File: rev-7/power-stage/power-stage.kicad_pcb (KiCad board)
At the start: 6 copper layers, 40 x 39.5 mm, 102 parts, among them J1 10132797-021100LF, J2 10132797-021100LF, J3 10132797-021100LF, J4 Motor, Q1 LMG5200, Q2 LMG5200, Q3 LMG5200, U1 AS5047P, U2 INA240A1PW, U3 INA240A1PW, U4 INA240A1PW

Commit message: Updating
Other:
- board text added: "Cutout GND plane under SW nodes"
- board text added: "F.Cu -> Sig In1.Cu -> PGND In2.Cu -> VBUS / sig In3.Cu -> Analog Sig In4.Cu -> PGND/GND B.Cu -> Phase/Sig"
- board text added: "Layer stackup: OSHPark 6-L 1oz copper -- 0.11mm prepreg -- 0.5oz copper -- 0.10mm prepreg -- 0.50oz copper -- 0.92mm core -- 0.5oz copper -- 0.10mm prepreg -- 0.5oz copper -- 0.11mm prepreg -- 1oz copper"
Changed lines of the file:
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@@
     (fp_line (start -15.000001 13.723079) (end -15.000001 13.435892) (layer "B.Mask") (width 0.1))
     (fp_line (start -14.000001 -14.276921) (end -16.890983 -14.276922) (layer "B.Mask") (width 0.1))
-    (fp_arc (start 16.890992 -14.276909) (mid 17.013752 -14.119771) (end 17.114589 -13.947741) (layer "B.Mask") (width 0.1))
+    (fp_arc (start 16.890992 -14.276909) (mid 17.013756 -14.119774) (end 17.114589 -13.947741) (layer "B.Mask") (width 0.1))
     (fp_arc (start -17.114591 -13.947741) (mid -17.013752 -14.11978) (end -16.890983 -14.276922) (layer "B.Mask") (width 0.1))
     (fp_arc (start -14.000001 14.723079) (mid -14.707108 14.430186) (end -15.000001 13.723079) (layer "B.Mask") (width 0.1))
@@
       (connect_pads (clearance 0))
       (min_thickness 0.254)
-      (keepout (tracks allowed) (vias allowed) (pads not_allowed ) (copperpour allowed) (footprints not_allowed))
+      (keepout (tracks allowed) (vias allowed) (pads not_allowed) (copperpour allowed) (footprints not_allowed))
       (fill (thermal_gap 0.508) (thermal_bridge_width 0.508))
       (polygon
@@
       (connect_pads (clearance 0))
       (min_thickness 0.254)
-      (keepout (tracks allowed) (vias allowed) (pads not_allowed ) (copperpour allowed) (footprints not_allowed))
+      (keepout (tracks allowed) (vias allowed) (pads not_allowed) (copperpour allowed) (footprints not_allowed))
       (fill (thermal_gap 0.508) (thermal_bridge_width 0.508))
       (polygon
@@
     )
   )
+  (gr_text "Layer stackup:\nOSHPark 6-L\n1oz copper\n-- 0.11mm prepreg --\n0.5oz copper\n-- 0.10mm prepreg --\n0.50oz copper\n-- 0.92mm core -- \n0.5oz copper \n-- 0.10mm prepreg --\n0.5oz copper\n-- 0.11mm prepreg --\n1oz copper" (at 128.15 51.45) (layer "Cmts.User")
+    (effects (font (size 0.5 0.5) (thickness 0.1)))
+  )
   (gr_text "1.65mm Clearance Zone" (at 97.475 62.425) (layer "Cmts.User")
     (effects (font (size 0.6 0.6) (thickness 0.15)))
   )
+  (gr_text "F.Cu -> Sig\nIn1.Cu -> PGND\nIn2.Cu -> VBUS / sig\nIn3.Cu -> Analog Sig\nIn4.Cu -> PGND/GND\nB.Cu -> Phase/Sig" (at 125.65 67.4) (layer "Cmts.User")
+    (effects (font (size 0.5 0.5) (thickness 0.1)))
+  )
+  (gr_text "Cutout GND plane under SW nodes" (at 127.2 74.4) (layer "Cmts.User")
+    (effects (font (size 0.5 0.5) (thickness 0.1)))
+  )
   (zone (net 43) (net_name "/PHA_RAW") (layer "F.Cu") (hatch edge 0.508)

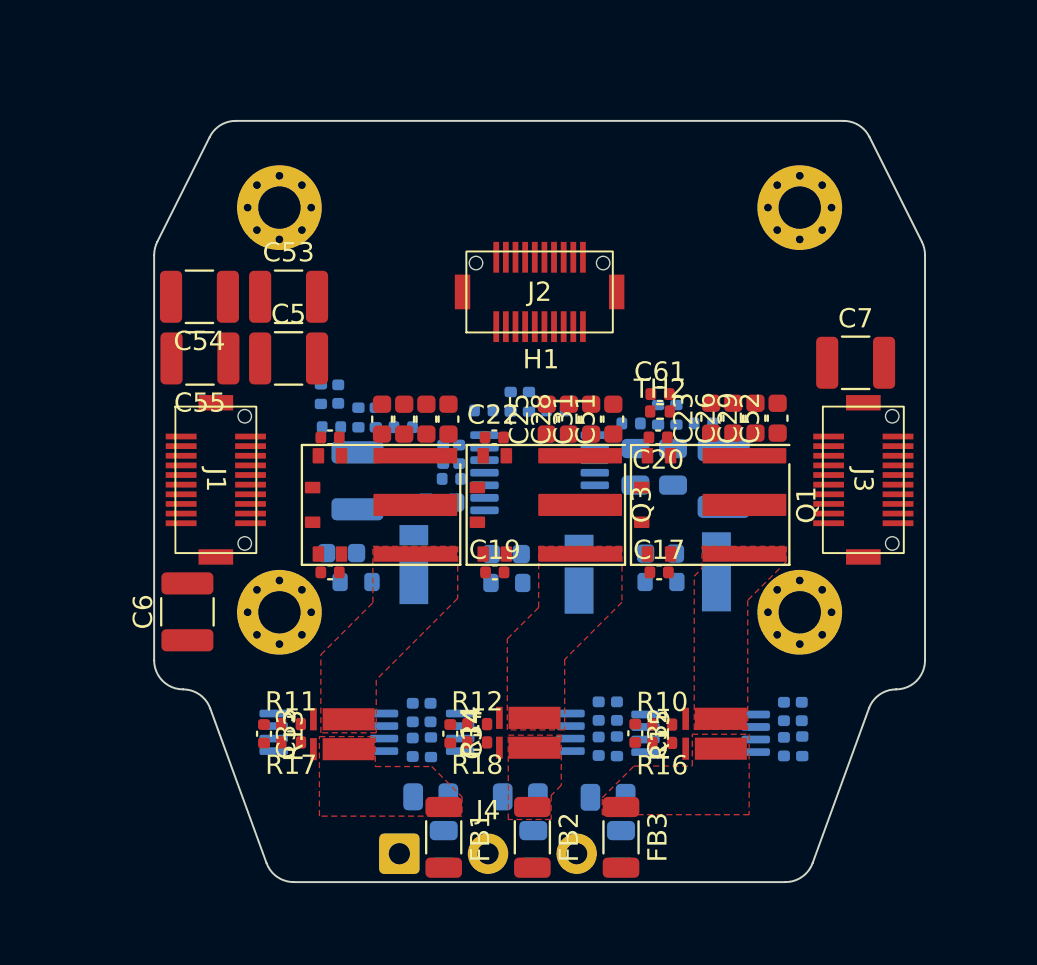
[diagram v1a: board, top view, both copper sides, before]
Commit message: Rev 7 RC1 - Push before design review
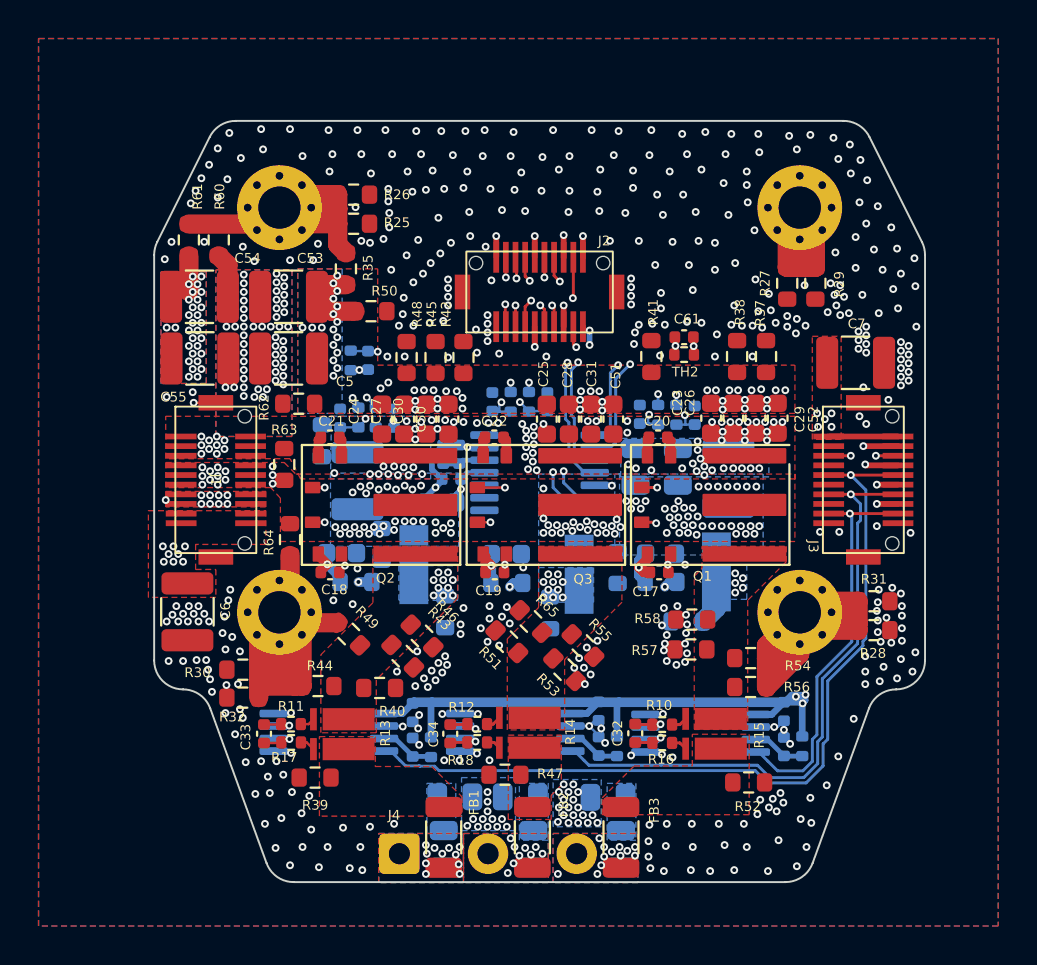
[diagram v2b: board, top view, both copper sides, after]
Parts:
- removed C44, C45, C46: 2.2u, Capacitor_SMD:C_0402_1005Metric
- added R25: THJP0603ABT1, Resistor_SMD:R_0603_1608Metric, F.Cu at (87.7, 54.5)
- added R26: THJP0603ABT1, Resistor_SMD:R_0603_1608Metric, F.Cu at (87.7, 53.0)
- added R27: THJP0603ABT1, Resistor_SMD:R_0603_1608Metric, F.Cu at (110.2, 57.5)
- added R28: THJP0603ABT1, Resistor_SMD:R_0603_1608Metric, F.Cu at (114.7, 75.5)
- added R29: THJP0603ABT1, Resistor_SMD:R_0603_1608Metric, F.Cu at (111.6, 57.5)
- added R30: THJP0603ABT1, Resistor_SMD:R_0603_1608Metric, F.Cu at (81.9, 77.6)
- added R31: THJP0603ABT1, Resistor_SMD:R_0603_1608Metric, F.Cu at (114.7, 74.0)
- added R32: THJP0603ABT1, Resistor_SMD:R_0603_1608Metric, F.Cu at (81.9, 79.0)
- added R33: THJP0603ABT1, Resistor_SMD:R_0603_1608Metric, B.Cu at (89.1, 71.1)
- added R34: THJP0603ABT1, Resistor_SMD:R_0603_1608Metric, B.Cu at (86.0, 65.7)
- added R35: THJP0603ABT1, Resistor_SMD:R_0603_1608Metric, F.Cu at (87.2, 56.8)
- added R36: THJP0603ABT1, Resistor_SMD:R_0603_1608Metric, B.Cu at (101.3, 72.3)
- added R37: THJP0603ABT1, Resistor_SMD:R_0603_1608Metric, F.Cu at (109.0, 61.4)
- added R38: THJP0603ABT1, Resistor_SMD:R_0603_1608Metric, F.Cu at (107.5, 61.4)
- added R39: THJP0603ABT1, Resistor_SMD:R_0603_1608Metric, F.Cu at (85.7, 83.2)
- added R40: THJP0603ABT1, Resistor_SMD:R_0603_1608Metric, F.Cu at (89.0, 78.5)
- added R41: THJP0603ABT1, Resistor_SMD:R_0603_1608Metric, F.Cu at (103.1, 61.4)
- added R42: THJP0603ABT1, Resistor_SMD:R_0603_1608Metric, F.Cu at (93.3, 61.4)
- added R43: THJP0603ABT1, Resistor_SMD:R_0603_1608Metric, F.Cu at (90.2, 76.9)
- added R44: THJP0603ABT1, Resistor_SMD:R_0603_1608Metric, F.Cu at (85.8, 78.5)
- added R45: THJP0603ABT1, Resistor_SMD:R_0603_1608Metric, F.Cu at (91.9, 61.4)
- added R46: THJP0603ABT1, Resistor_SMD:R_0603_1608Metric, F.Cu at (91.2, 75.8)
- added R47: THJP0603ABT1, Resistor_SMD:R_0603_1608Metric, F.Cu at (95.5, 83.0)
- added R48: THJP0603ABT1, Resistor_SMD:R_0603_1608Metric, F.Cu at (90.4, 61.4)
- added R49: THJP0603ABT1, Resistor_SMD:R_0603_1608Metric, F.Cu at (87.4, 75.8)
- added R50: THJP0603ABT1, Resistor_SMD:R_0603_1608Metric, F.Cu at (88.5, 59.0)
- added R51: THJP0603ABT1, Resistor_SMD:R_0603_1608Metric, F.Cu at (95.6, 76.2)
- added R52: THJP0603ABT1, Resistor_SMD:R_0603_1608Metric, F.Cu at (108.2, 83.5)
- added R53: THJP0603ABT1, Resistor_SMD:R_0603_1608Metric, F.Cu at (98.6, 77.6)
- added R54: THJP0603ABT1, Resistor_SMD:R_0603_1608Metric, F.Cu at (108.2, 77.0)
- added R55: THJP0603ABT1, Resistor_SMD:R_0603_1608Metric, F.Cu at (99.5, 76.3)
- added R56: THJP0603ABT1, Resistor_SMD:R_0603_1608Metric, F.Cu at (108.2, 78.5)
- added R57: THJP0603ABT1, Resistor_SMD:R_0603_1608Metric, F.Cu at (105.2, 76.5)
- added R58: THJP0603ABT1, Resistor_SMD:R_0603_1608Metric, F.Cu at (105.2, 75.0)
- added R59: THJP0603ABT1, Resistor_SMD:R_0603_1608Metric, B.Cu at (105.0, 75.1)
- added R60: THJP0603ABT1, Resistor_SMD:R_0603_1608Metric, F.Cu at (80.7, 55.3)
- added R61: THJP0603ABT1, Resistor_SMD:R_0603_1608Metric, F.Cu at (79.1, 55.3)
- added R62: THJP0603ABT1, Resistor_SMD:R_0603_1608Metric, F.Cu at (84.8, 63.8)
- added R63: THJP0603ABT1, Resistor_SMD:R_0603_1608Metric, F.Cu at (84.0, 67.0)
- added R64: THJP0603ABT1, Resistor_SMD:R_0603_1608Metric, F.Cu at (84.3, 70.8)
- added R65: THJP0603ABT1, Resistor_SMD:R_0603_1608Metric, F.Cu at (96.8, 75.1)
- added R66: THJP0603ABT1, Resistor_SMD:R_0603_1608Metric, B.Cu at (92.4, 74.6)
- added R67: THJP0603ABT1, Resistor_SMD:R_0603_1608Metric, B.Cu at (97.8, 74.7)
- C28, C31: value 4.7u -> 10u
- R13, R14, R15: value 10m -> 9m
- moved TH2 3.20 mm to (104.8, 61.2)
- moved C61 3.20 mm to (104.8, 60.4)
- moved C60 2.34 mm to (88.4, 61.5)
- moved TH1 2.34 mm to (87.5, 61.5)
- moved R24 1.25 mm to (92.9, 84.2), turned to 0 degrees
- moved C12 0.66 mm to (89.8, 64.5), turned to 90 degrees
- moved C14 0.65 mm to (102.5, 64.3), turned to 90 degrees
- moved C15 0.65 mm to (87.0, 64.5), turned to 90 degrees
- moved C13 0.64 mm to (97.7, 63.7), turned to 90 degrees
- moved C16 0.64 mm to (94.8, 63.7), turned to 90 degrees
- moved C11 0.62 mm to (105.3, 64.4), turned to 90 degrees
- moved C36 0.25 mm to (107.1, 67.7)
- moved C37 0.25 mm to (104.5, 67.1)
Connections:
- R22 pad 2: PWRGND -> PGND
- R23 pad 2: PWRGND -> PGND
- R24 pad 2: PWRGND -> PGND
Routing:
- net /CHASSIS: track 0.00 -> 74.8 mm
- net /IA_SNS: track 0.00 -> 43.8 mm, vias 0 -> 1
- net /THERM_A: track 0.00 -> 40.0 mm, vias 0 -> 2
- net +3V3A: track 0.00 -> 39.0 mm, vias 0 -> 8
- net GND: track 0.00 -> 34.4 mm, vias 0 -> 447
- net /IB_SNS: track 0.00 -> 32.4 mm, vias 0 -> 1
- net /IC_SNS: track 0.00 -> 20.9 mm, vias 0 -> 1
- net /THERM_B: track 0.00 -> 15.5 mm, vias 0 -> 2
- net /ENC_B: track 0.00 -> 15.1 mm, vias 0 -> 2
- net /SPI_SCK: track 0.00 -> 14.4 mm, vias 0 -> 2
- net /PHC_L: track 0.00 -> 13.7 mm, vias 0 -> 2
- net /PHC_H: track 0.00 -> 12.9 mm, vias 0 -> 2
- net /SPI_nCS: track 0.00 -> 12.4 mm, vias 0 -> 2
- net /ENC_A: track 0.00 -> 12.1 mm, vias 0 -> 2
- net /PHA_H: track 0.00 -> 12.1 mm, vias 0 -> 2
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- added copper zone on F.Cu, net +3V3A
- added copper zone on In3.Cu, net +3V3A
- added copper zone on F.Cu, net +5V
- added copper zone on In3.Cu, net +5V
- added copper zone on B.Cu, net /PHA_FLT
- added copper zone on F.Cu, net /PHA_FLT
- added copper zone on B.Cu, net /PHA_RAW
- added copper zone on B.Cu, net /PHB_FLT
- added copper zone on F.Cu, net /PHB_FLT
- added copper zone on B.Cu, net /PHB_RAW
- added copper zone on B.Cu, net /PHC_FLT
- added copper zone on F.Cu, net /PHC_FLT
- added copper zone on B.Cu, net /PHC_RAW
- added copper zone on B.Cu, net GND
- added copper zone on F.Cu, net GND
- added copper zone on In1.Cu, net GND
- added copper zone on In2.Cu, net GND
- added copper zone on In3.Cu, net GND
- added copper zone on In4.Cu, net GND
- added copper zone on B.Cu, net Net-(C47-Pad2)
- added copper zone on B.Cu, net Net-(C48-Pad2)
- added copper zone on B.Cu, net Net-(C49-Pad2)
- added copper zone on B.Cu, net PGND
- added copper zone on F.Cu, net PGND
- added copper zone on In1.Cu, net PGND
- added copper zone on B.Cu, net VBUS
- added copper zone on F.Cu, net VBUS
- added copper zone on In2.Cu, net VBUS
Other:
- board text added: "F.Cu -> PWR In1.Cu -> PGND In2.Cu -> VBUS In3.Cu -> Sig In4.Cu -> GND B.Cu -> Analog/Sig"
- board text removed: "F.Cu -> Sig In1.Cu -> PGND In2.Cu -> VBUS / sig In3.Cu -> Analog Sig In4.Cu -> PGND/GND B.Cu -> Phase/Sig"
